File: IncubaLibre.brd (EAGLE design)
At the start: 100 x 55.9 mm, 22 parts, among them T1 P-MOSFET

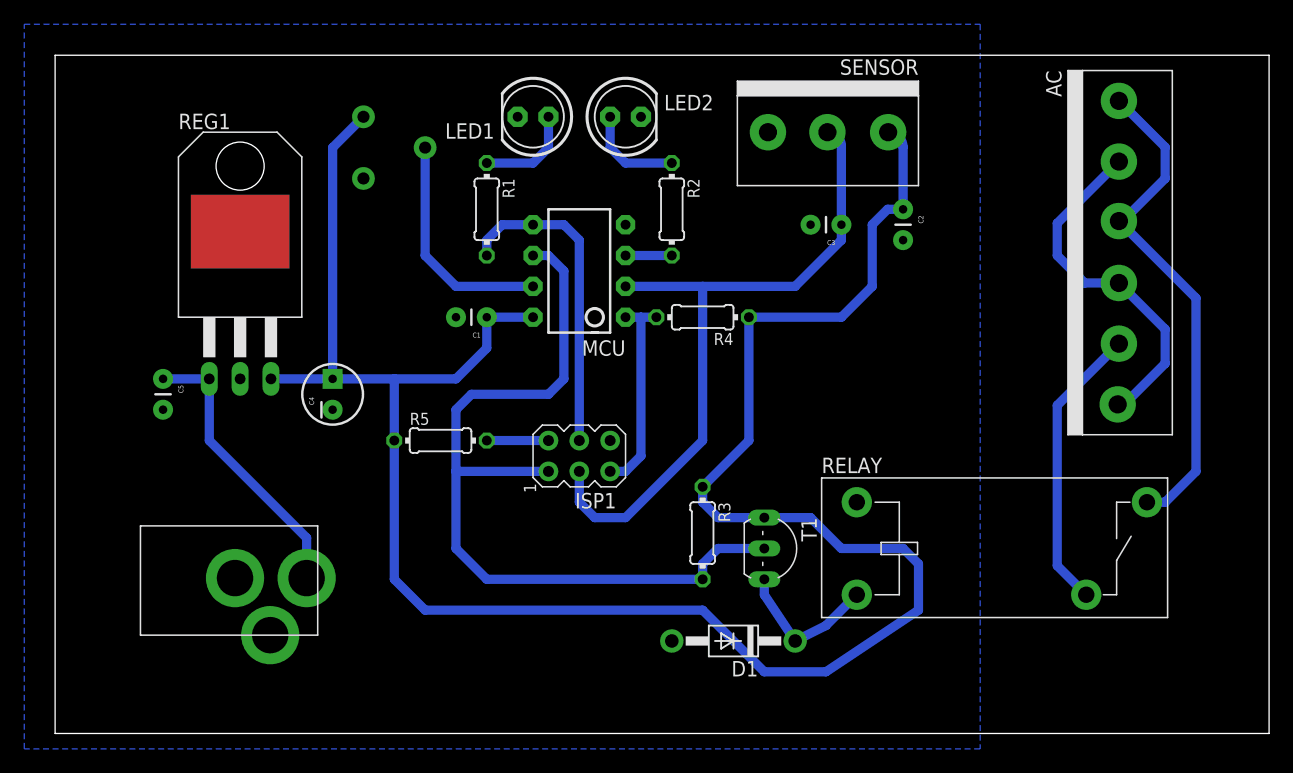
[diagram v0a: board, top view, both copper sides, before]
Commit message: Initial buggy firmware code.
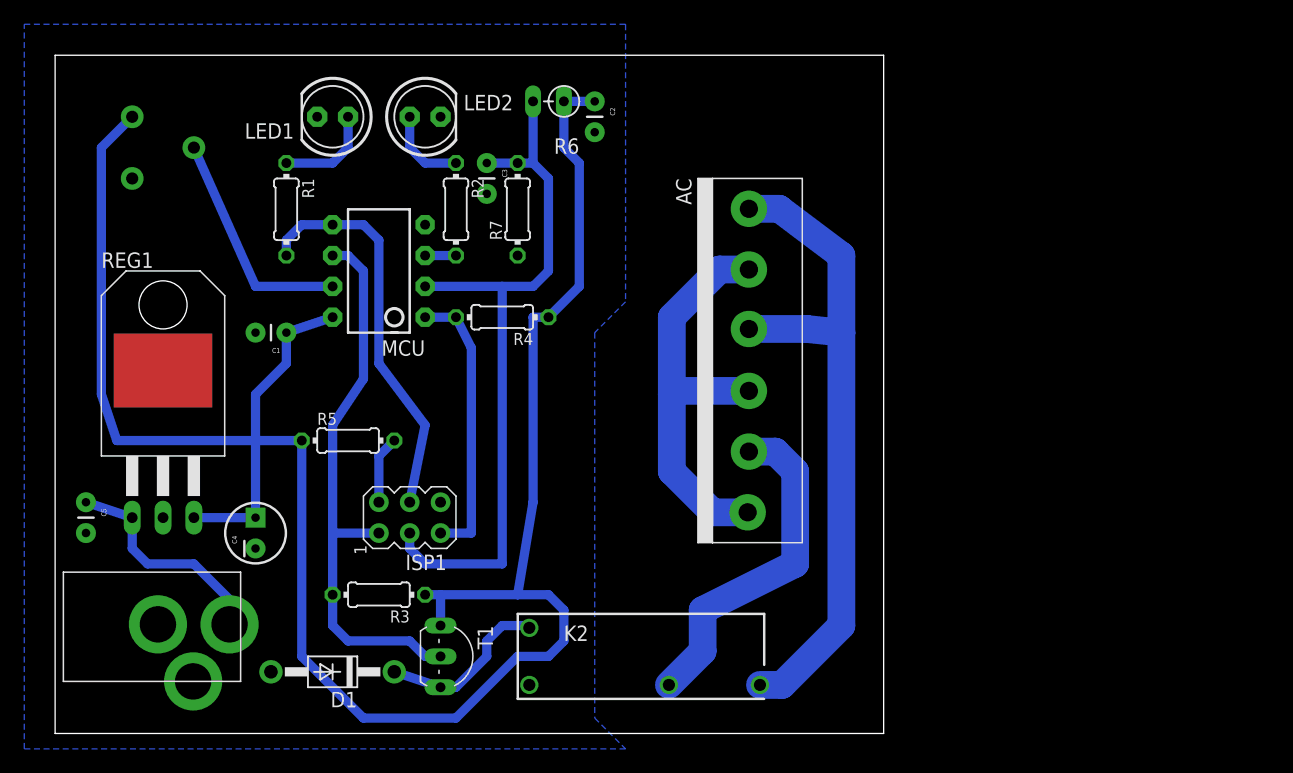
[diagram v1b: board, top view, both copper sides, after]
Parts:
- removed RELAY: RELAY-SPST-NO, Robin:G6RL-1A-DC3
- removed SENSOR: TERMINAL-3, Robin:MBE-153
- added K2: LD14H, relay:LD
- added R6: THERMISTOR-2,5, varistor:RS-2,5
- added R7: 1.5K, resistor:0204/7
- moved D1 33.1 mm to (22.9, 5.08)
- moved AC 31.8 mm to (57.1, 45.7)
- moved C3 29.6 mm to (35.6, 47.0), turned to 270 degrees
- moved T1 28.1 mm to (31.8, 6.35)
- moved R3 27.1 mm to (26.7, 11.4), turned to 180 degrees
- moved C2 26.9 mm to (44.5, 52.1)
- moved POT 19.0 mm to (6.35, 48.3)
- moved R2 17.8 mm to (33.0, 43.2)
- moved C1 16.6 mm to (19.1, 33.0)
- moved R4 16.5 mm to (36.8, 34.3)
- moved LED2 16.5 mm to (30.5, 50.8)
- moved R1 16.5 mm to (19.1, 43.2)
- moved LED1 16.5 mm to (22.9, 50.8)
- moved MCU 16.5 mm to (26.7, 38.1)
- moved ISP1 14.9 mm to (29.2, 17.8)
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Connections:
- net AC1: now also K2.NO; no longer RELAY.3
- net AC1_REL: now also K2.COM; no longer RELAY.2
- net GND: now also K2.2, R7.1; no longer RELAY.5, SENSOR.3
- net T1: now also K2.1; no longer RELAY.1
- net TEMP: now also R6.2, R7.2; no longer SENSOR.2
- net VCC: now also R6.1; no longer SENSOR.1
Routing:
- net RELAY: track 69.2 -> 46.8 mm
- net AC1: track 41.6 -> 55.8 mm
- net LED1: track 26.5 -> 32.9 mm
- net RST: track 17.0 -> 23.2 mm
- net AC2: track 29.4 -> 34.8 mm
- net N$9: track 23.5 -> 18.4 mm
- net AC1_REL: track 23.8 -> 27.9 mm
- net TEMP: track 57.3 -> 61.3 mm
- net VCC: track 178.9 -> 175.8 mm
- net T1: track 12.3 -> 14.3 mm
- net N$5: track 8.15 -> 6.88 mm
- net LED2: track 3.81 -> 2.54 mm
- net N$1: track 5.08 -> 5.61 mm
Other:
- board size 100 x 55.9 mm -> 68.2 x 55.9 mm
